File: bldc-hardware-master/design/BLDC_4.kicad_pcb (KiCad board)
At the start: 4 copper layers, 48.4 x 75 mm, 132 parts, among them J1 7466103, J2 7466103, J3 7466103, J4 7466103, J5 7466103, K1 SERVO, P1 HALL/Encoder, P101 CANBUS, P2 SWD, P3 PWR_COMM, P4 IN+, P5 IN-, P6 MOTOR1, P7 MOTOR2, P9 MOTOR3, Q1 IRFS7530, Q2 IRFS7530, Q3 IRFS7530, Q4 IRFS7530, Q5 IRFS7530, Q6 IRFS7530, U1 STM32F40X_LQFP64, U2 TC2117, U3 DRV8302, U401 SN65HVD232, X1 MINI-USB-SHIELD-32005-201, X2 8MHz 10ppm

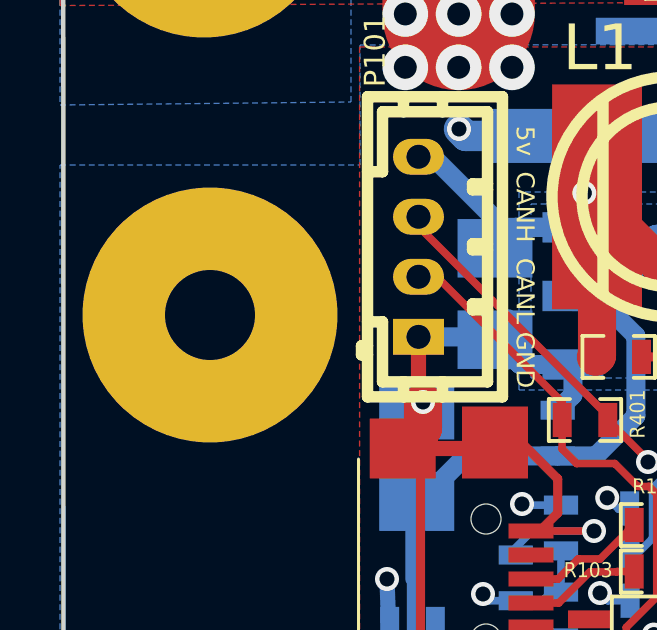
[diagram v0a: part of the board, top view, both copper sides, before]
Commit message: changes
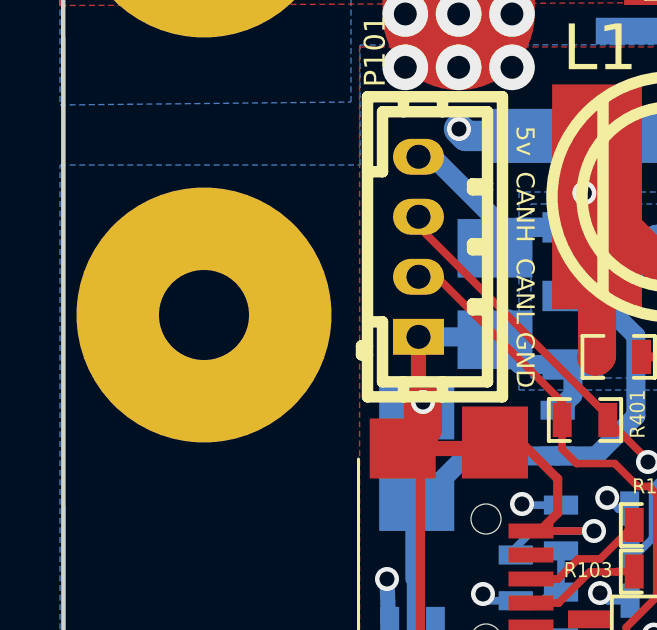
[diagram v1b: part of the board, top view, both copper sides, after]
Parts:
- moved J5 0.20 mm to (73.3, 119.0)
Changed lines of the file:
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@@
 	(footprint "vesc:7466103"
 		(layer "B.Cu")
-		(at 73.5 119 180)
+		(at 73.3 119 180)
 		(descr "7466103-3")
 		(tags "Connector")
